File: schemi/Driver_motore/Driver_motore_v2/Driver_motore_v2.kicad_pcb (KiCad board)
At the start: 2 copper layers, 173 x 113 mm, 38 parts, among them J1 PICKIT, J2 Motore, J3 Power, J4 Conn, J5 controllo_motore, J6 controllo_encoder, J7 controllo_alimentazione, U1 L298N, U2 PIC16F88-IP, U3 LM7805_TO220

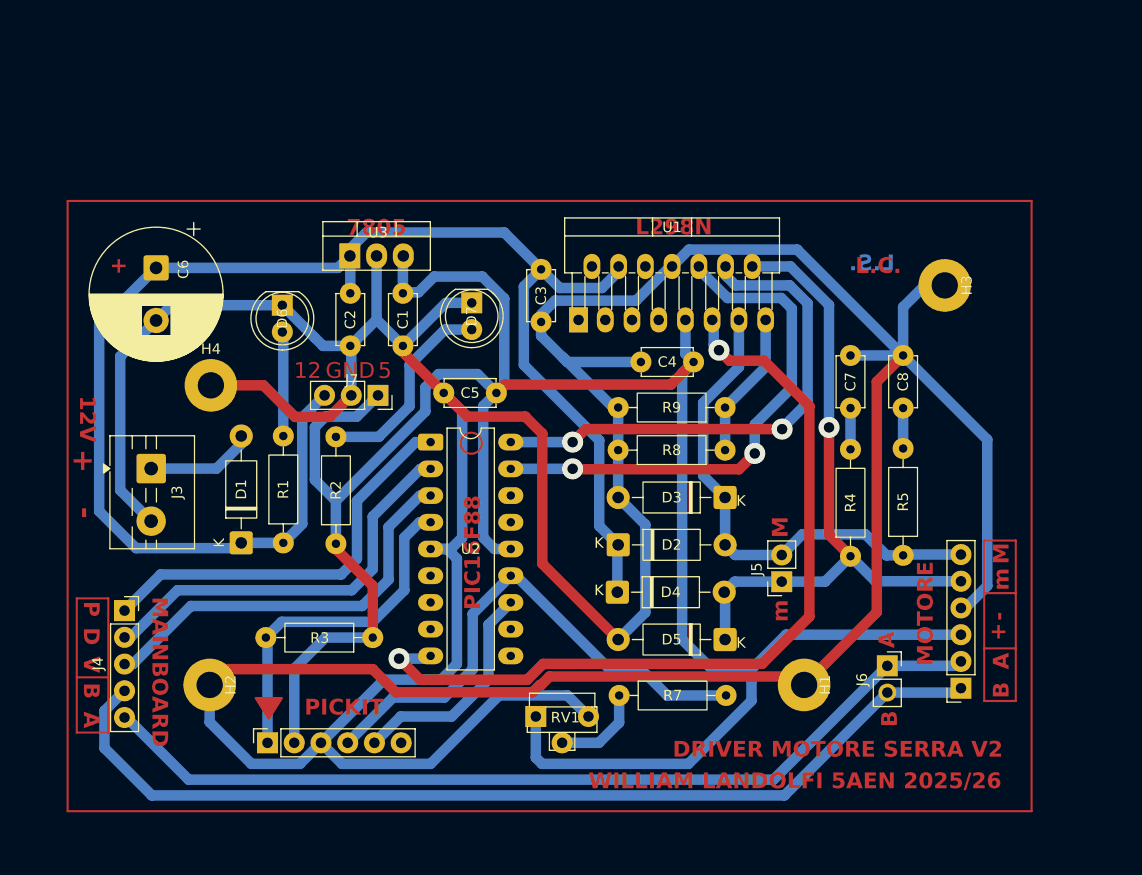
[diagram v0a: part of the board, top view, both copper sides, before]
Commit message: update main board
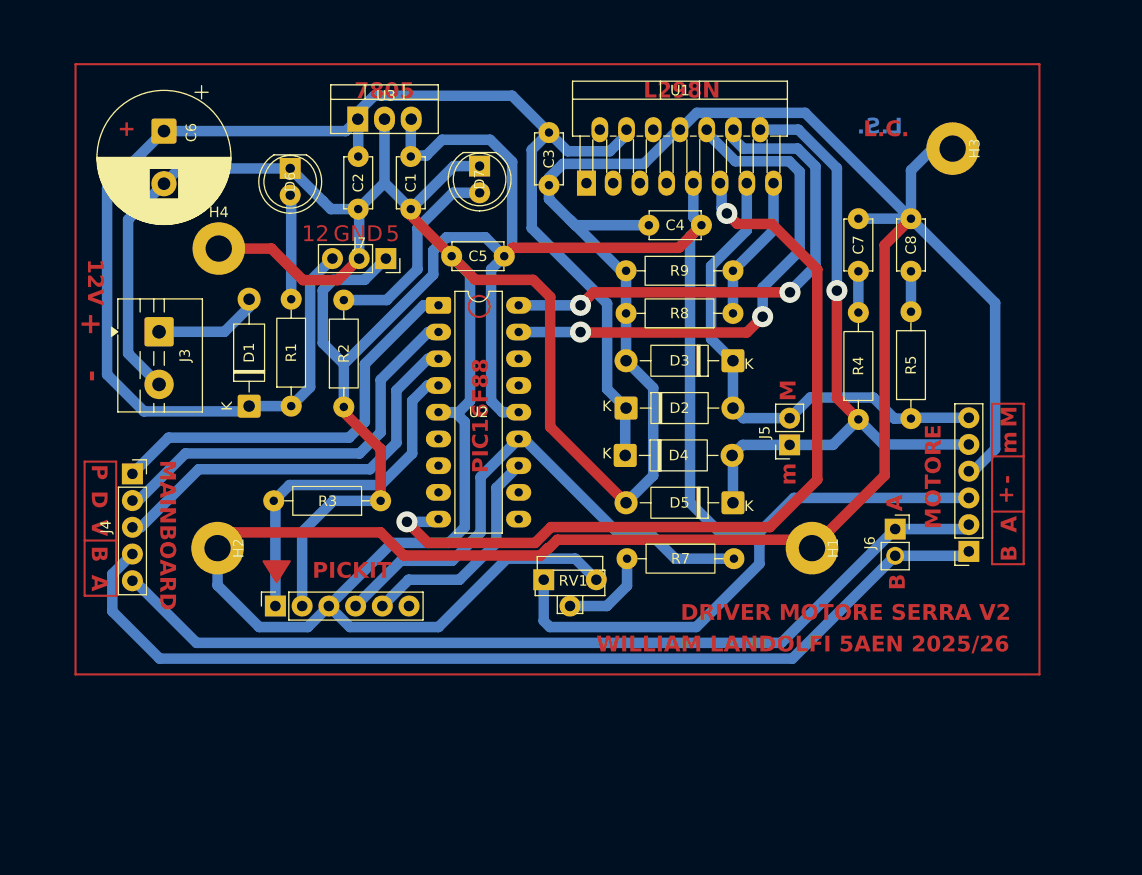
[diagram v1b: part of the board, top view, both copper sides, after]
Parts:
- moved J5 13.0 mm to (128.1, 71.7)
- moved C1 13.0 mm to (92.1, 49.3)
- moved C2 13.0 mm to (87.1, 44.3)
- moved C3 13.0 mm to (105.2, 47.0)
- moved C4 13.0 mm to (119.7, 50.8)
- moved C5 13.0 mm to (96.0, 53.8)
- moved C6 13.0 mm to (68.7, 41.9)
- moved D1 13.0 mm to (76.8, 68.0)
- moved D2 13.0 mm to (112.6, 68.2)
- moved D4 13.0 mm to (112.5, 72.7)
- moved D5 13.0 mm to (122.7, 77.2)
- moved D6 13.0 mm to (80.7, 45.4)
- moved D7 13.0 mm to (98.7, 45.2)
- moved H1 13.0 mm to (130.2, 81.5)
- moved H2 13.0 mm to (73.8, 81.5)
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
